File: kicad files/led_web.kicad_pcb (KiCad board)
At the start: 2 copper layers, 40 x 60 mm, 5 parts, among them U1 MAX4466, U2 WeMos_D1_mini, U3 SSD1306

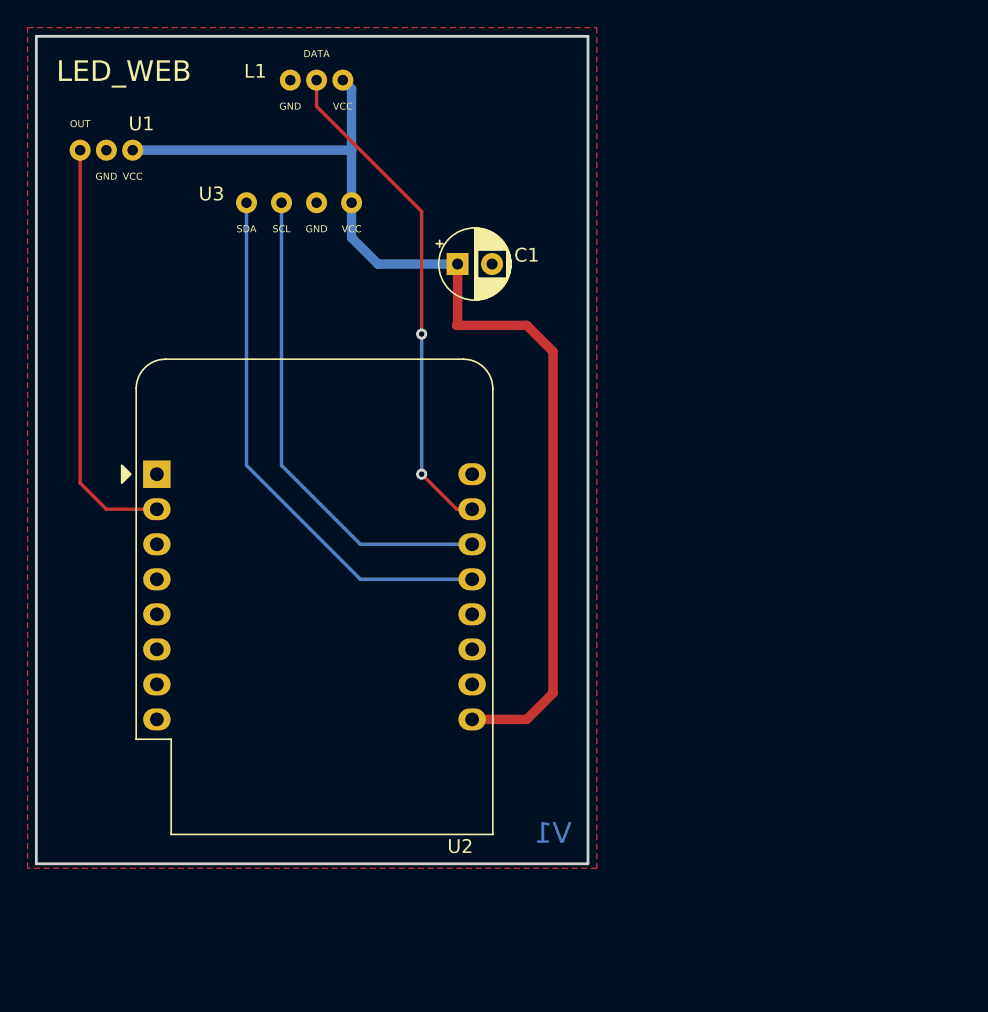
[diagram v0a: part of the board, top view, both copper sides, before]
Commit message: pcb redesign
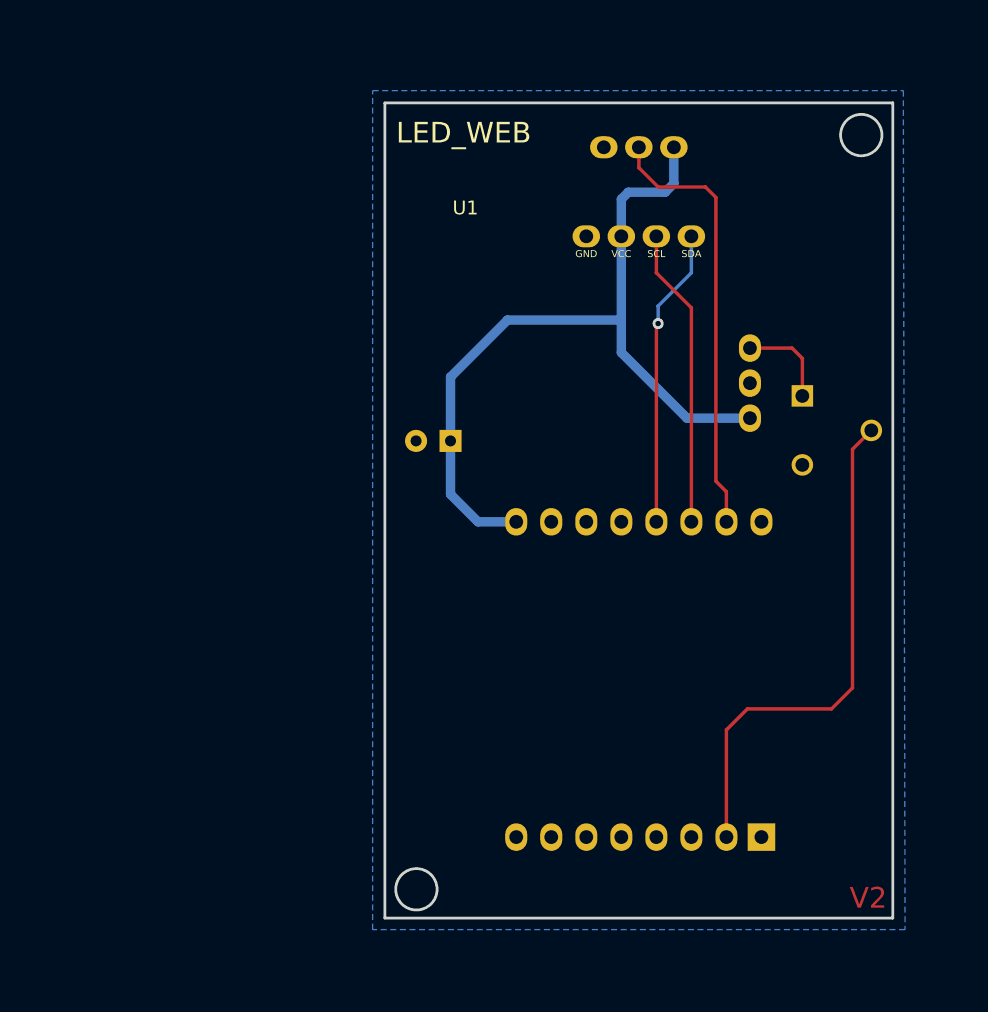
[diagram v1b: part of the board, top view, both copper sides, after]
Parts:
- added RV1: R_Potentiometer, Potentiometer_THT:Potentiometer_Runtron_RM-065_Vertical, B.Cu at (163.5, 78.8)
- C1, L1, U2: moved to B.Cu
- U1: value MAX4466 -> SSD1306; footprint led_web_foots:MAX4466 -> led_web_foots:SSD1306
- U3: value SSD1306 -> MAX4466; footprint led_web_foots:SSD1306 -> led_web_foots:MAX4466; moved to B.Cu
- moved U2 51.1 mm to (160.5, 110.8), turned to 90 degrees
- moved U1 38.9 mm to (151.6, 65.9)
- moved U3 36.4 mm to (161.0, 77.9), turned to 90 degrees
- moved L1 23.9 mm to (151.6, 60.7)
- moved C1 12.8 mm to (138.0, 82.0), turned to 180 degrees
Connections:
- U1 pad 1: Net-(C1-Pad1) -> Net-(U1-Pad1)
- U1 pad 2: GND -> Net-(U1-Pad2)
- U1 pad 3: Net-(U1-Pad3) -> Net-(C1-Pad1)
- U2 pad 13: Net-(U1-Pad4) -> Net-(U1-Pad1)
- U2 pad 14: Net-(U1-Pad3) -> Net-(U1-Pad2)
- U2 pad 2: Net-(U2-Pad2) -> Net-(RV1-Pad2)
- U3 pad 1: Net-(C1-Pad1) -> Net-(RV1-Pad1)
- U3 pad 3: Net-(U2-Pad2) -> Net-(C1-Pad1)
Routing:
- net Net-(U1-Pad3): track 65.7 -> 0.00 mm
- net Net-(U1-Pad4): track 38.8 -> 0.00 mm
- net Net-(RV1-Pad2): track 0.00 -> 37.4 mm
- net Net-(C1-Pad1): track 79.7 -> 57.5 mm
- net Net-(U1-Pad2): track 0.00 -> 21.8 mm
- net Net-(U1-Pad1): track 0.00 -> 21.8 mm, vias 0 -> 1
- net Net-(RV1-Pad1): track 0.00 -> 6.84 mm
- net Net-(L1-Pad2): track 36.4 -> 31.8 mm, vias 2 -> 0
- added copper zone on B.Cu, net GND
- removed copper zone on F.Cu, net GND
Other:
- board size 40 x 60 mm -> 36.8 x 59.1 mm
- board text added: "V2"
- board text removed: "V1"
